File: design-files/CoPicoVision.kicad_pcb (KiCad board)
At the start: 2 copper layers, 33 parts, among them J301 DE15_Receptacle_HighDensity_M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, SW101 SW_Push, U101 Z80CPU, U102 DS1813, U103 74ACT05, U201 GAL22V10, U202 GAL22V10, U203 AT28C64, U204 AS6C6264, U301 Pico, U302 74LVC245, U303 74LVC245, X101 3.579545MHZ

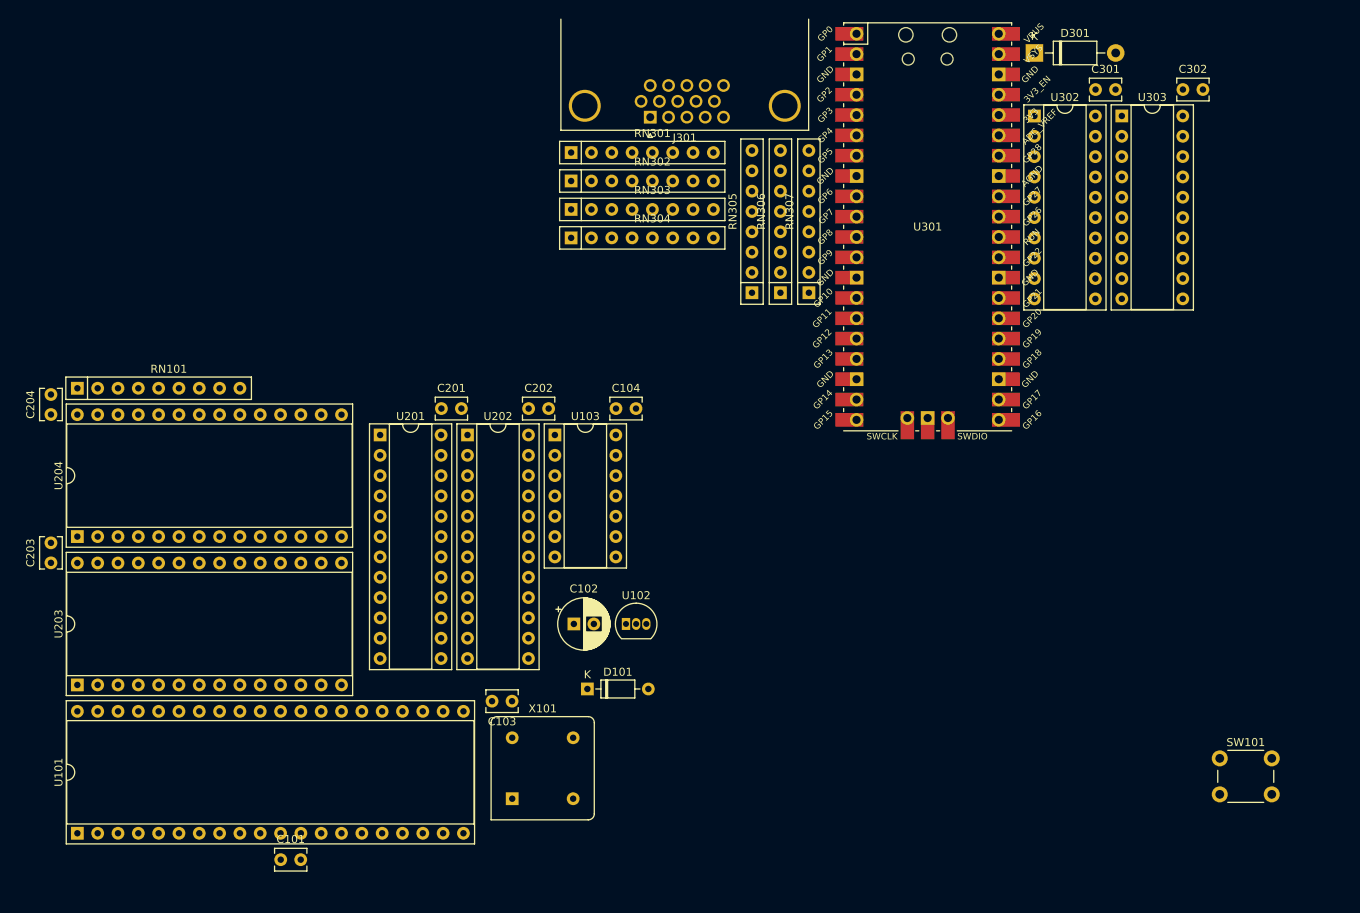
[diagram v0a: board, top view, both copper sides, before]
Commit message: Add controller ports just to get them onto the board.
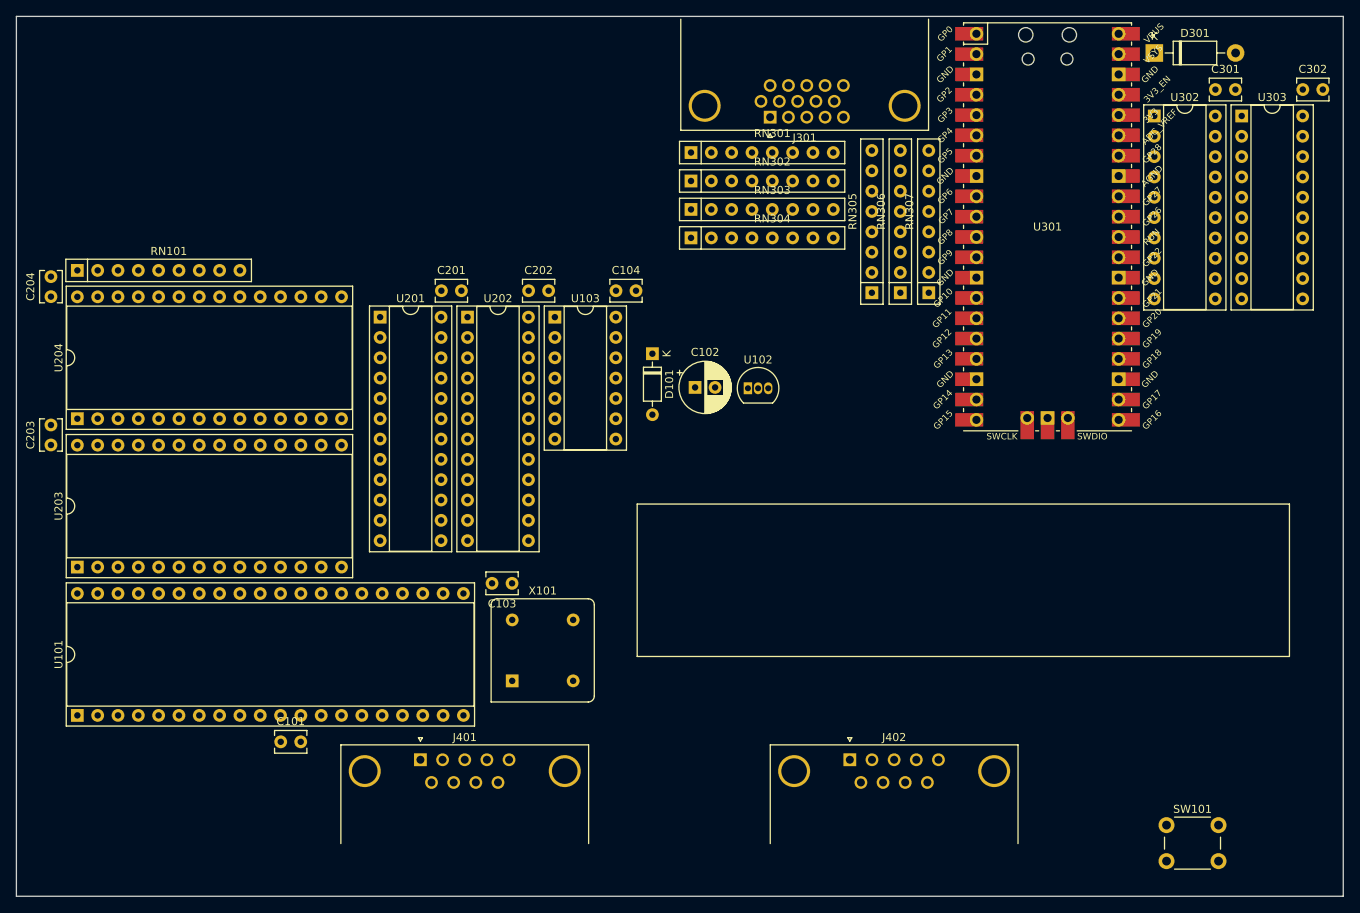
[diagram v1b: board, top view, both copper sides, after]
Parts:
- added J401: DE9_Plug_MountingHoles, Connector_Dsub:DSUB-9_Male_Horizontal_P2.77x2.84mm_EdgePinOffset7.70mm_Housed_MountingHolesOffset9.12mm, F.Cu at (91.7, 130.8)
- added J402: DE9_Plug_MountingHoles, Connector_Dsub:DSUB-9_Male_Horizontal_P2.77x2.84mm_EdgePinOffset7.70mm_Housed_MountingHolesOffset9.12mm, F.Cu at (145.3, 130.8)
- moved D101 42.7 mm to (120.7, 80.0), turned to -90 degrees
- moved C102 33.2 mm to (126.0, 84.2)
- moved U102 33.2 mm to (132.6, 84.3)
- moved D301 15.0 mm to (183.4, 42.4)
- moved J301 15.0 mm to (135.4, 50.4)
- moved RN306 15.0 mm to (151.6, 72.4)
- moved U302 15.0 mm to (183.4, 50.3)
- moved RN301 15.0 mm to (125.5, 54.9)
- moved RN302 15.0 mm to (125.5, 58.4)
- moved RN303 15.0 mm to (125.5, 62.0)
- moved RN304 15.0 mm to (125.5, 65.5)
- moved C301 15.0 mm to (191.0, 47.0)
- moved C302 15.0 mm to (201.9, 47.0)
- moved RN305 15.0 mm to (148.1, 72.4)
- moved RN307 15.0 mm to (155.2, 72.4)
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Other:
- board outline added: 165.9 x 110 mm
